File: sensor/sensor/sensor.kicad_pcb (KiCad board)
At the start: 4 copper layers, 60 x 21 mm, 61 parts, among them J1 RJ12_Shielded, J2 Conn_01x04, J3 Conn_01x06, J4 Conn_01x03_Socket, J5 Conn_01x03_Socket, J6 Conn_01x03_Socket, J7 Conn_01x03_Socket, SW5 SW_Coded_SH-7050, U1 PCA9615DP, U2 LTC4316xDD, U3 APDS-9960, U4 PCA9536DP, U5 TPS73101DBV, U6 ICM-20602, U7 VL53L1CXV0FY1

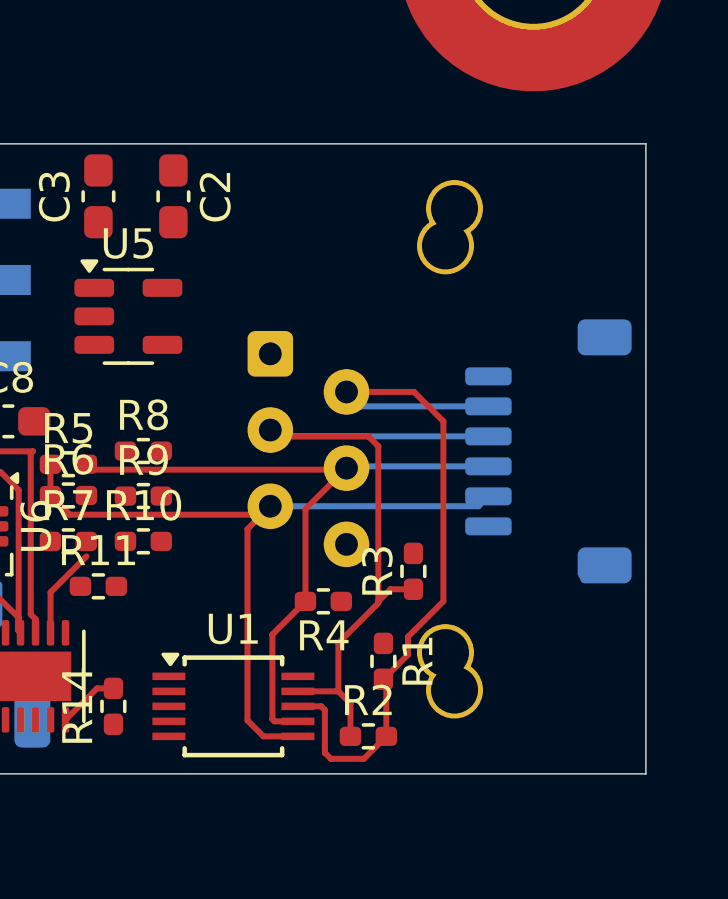
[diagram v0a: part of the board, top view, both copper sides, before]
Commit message: 3d models
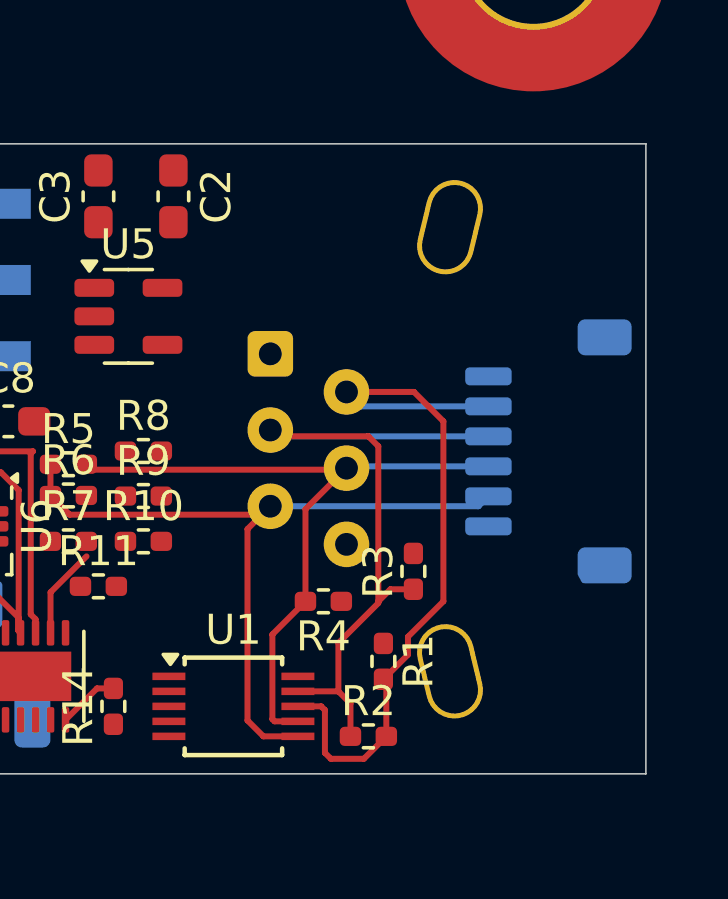
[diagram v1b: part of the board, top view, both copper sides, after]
